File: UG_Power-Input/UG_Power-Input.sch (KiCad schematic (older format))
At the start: 46 parts, among them J1 12V IN, J2 12V OUT, J3 5V OUT, U1 LM2679

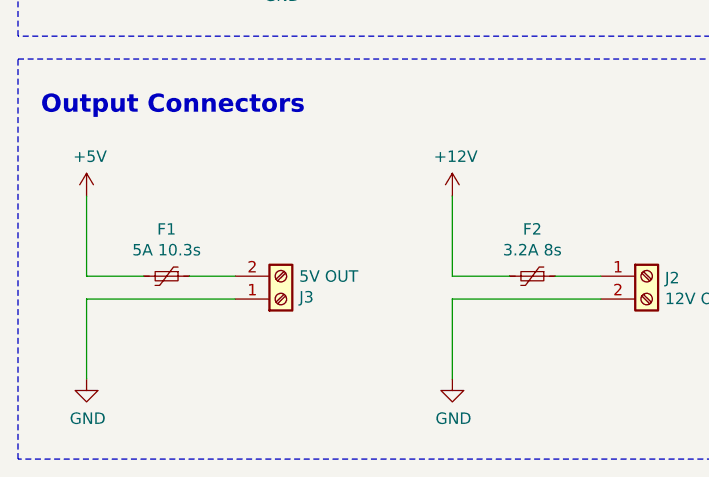
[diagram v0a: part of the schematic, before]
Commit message: Changes to PCB & BOM
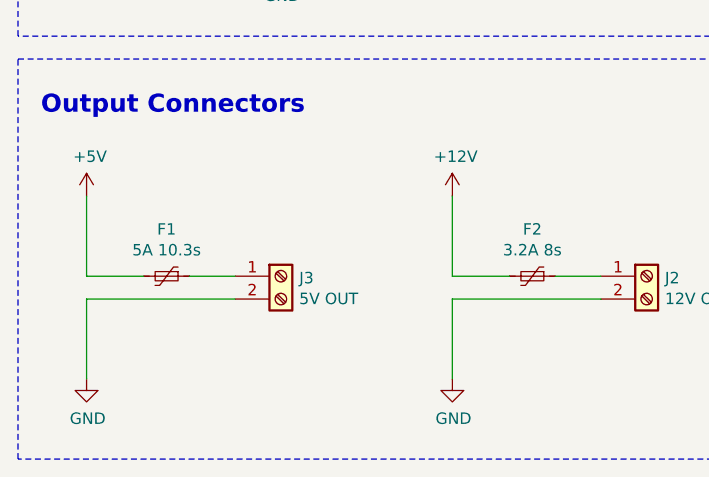
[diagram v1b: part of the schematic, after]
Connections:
- net GND: now also J3.2 (Pin_2); no longer J3.1 (Pin_1)
- net at F1.1: now also J3.1 (Pin_1); no longer J3.2 (Pin_2)
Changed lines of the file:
@@
 L Connector:Screw_Terminal_01x02 J3
 U 1 1 60791571
-P 2400 7000
+P 2400 6900
 AR Path="/60791571" Ref="J3"  Part="1"
 AR Path="/603AD409/60791571" Ref="J?"  Part="1"
@@
 AR Path="/6081FDFC/60597F98/60791571" Ref="J?"  Part="1"
 AR Path="/60599E1F/605B3C0B/60791571" Ref="J?"  Part="1"
-F 0 "J3" H 2480 6992 50  0000 L CNN
-F 1 "5V OUT" H 2480 6901 50  0000 L CNN
-F 2 "TerminalBlock_Phoenix:TerminalBlock_Phoenix_MKDS-1,5-2-5.08_1x02_P5.08mm_Horizontal" H 2400 7000 50  0001 C CNN
-F 3 "" H 2400 7000 50  0001 C CNN
-F 4 "" H 2400 7000 50  0001 C CNN "Manufacturer"
-F 5 "" H 2400 7000 50  0001 C CNN "Part-Nr."
-F 6 "~" H 2400 7000 50  0001 C CNN "Mouser-Nr"
-	1    2400 7000
-	1    0    0    1
+F 0 "J3" H 2480 6892 50  0000 L CNN
+F 1 "5V OUT" H 2480 6801 50  0000 L CNN
+F 2 "TerminalBlock_Phoenix:TerminalBlock_Phoenix_MKDS-1,5-2-5.08_1x02_P5.08mm_Horizontal" H 2400 6900 50  0001 C CNN
+F 3 "" H 2400 6900 50  0001 C CNN
+F 4 "" H 2400 6900 50  0001 C CNN "Manufacturer"
+F 5 "" H 2400 6900 50  0001 C CNN "Part-Nr."
+F 6 "~" H 2400 6900 50  0001 C CNN "Mouser-Nr"
+	1    2400 6900
+	1    0    0    -1
 $EndComp
 $Comp
